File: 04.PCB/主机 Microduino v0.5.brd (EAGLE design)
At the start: 50.8 x 50 mm, 22 parts

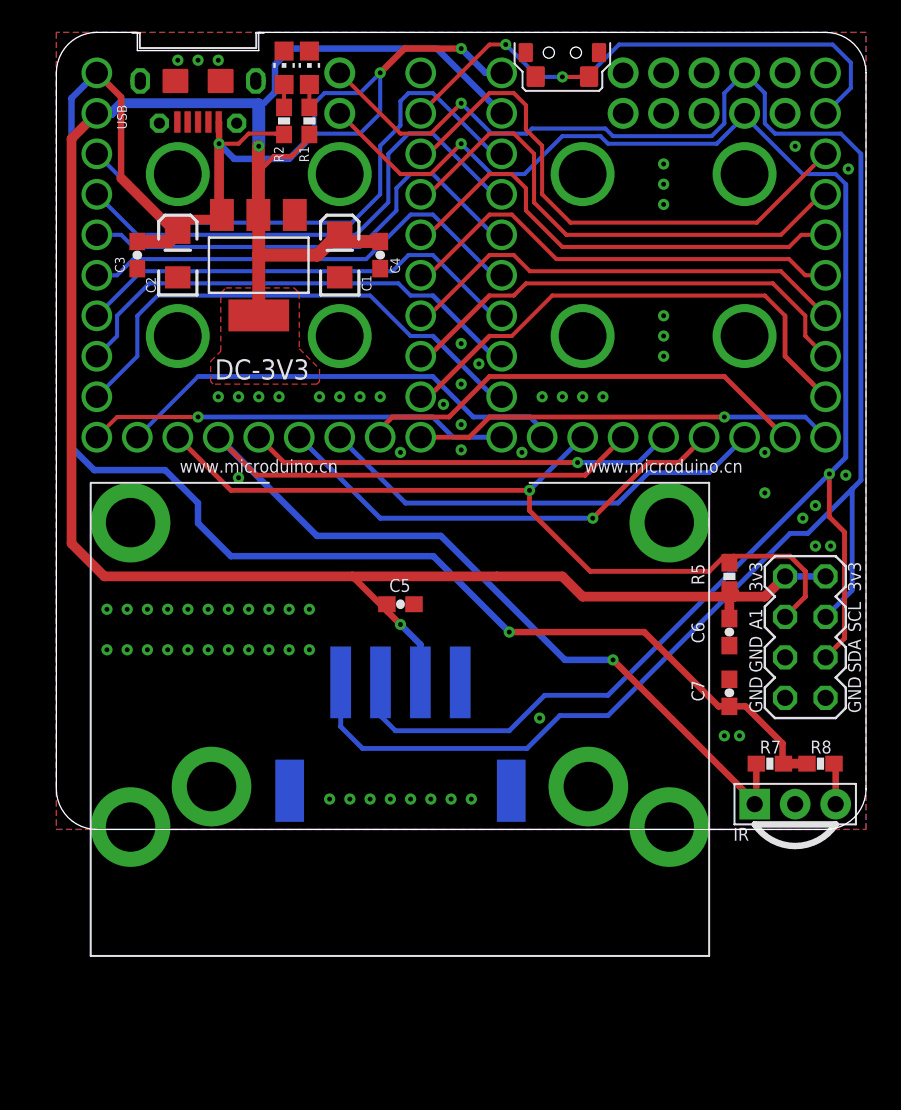
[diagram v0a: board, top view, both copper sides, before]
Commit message: 更新
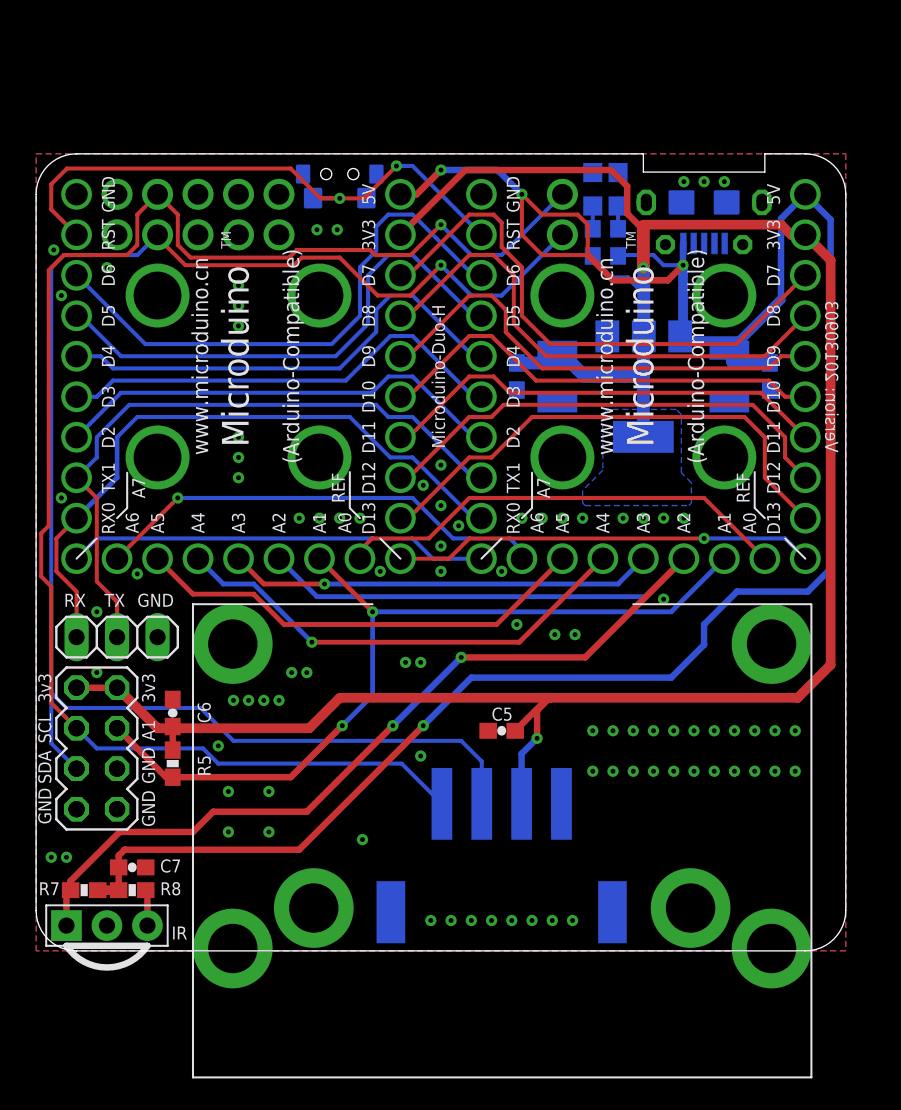
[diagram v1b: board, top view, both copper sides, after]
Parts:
- added JP2: (no value), pinhead:1X03
- added SV1: (no value), pkj:MA04-2
- C1, C2: device microduino:EIA3216 -> microduino:EIA3528
- moved SV2 45.0 mm to (5.71, 15.4), flipped to the bottom
- moved R8 43.9 mm to (7.94, 6.51)
- moved IR 43.8 mm to (6.35, 4.29)
- moved R7 43.7 mm to (4.92, 6.51)
- moved C3 40.4 mm to (47.9, 38.7), flipped to the bottom
- moved C7 39.0 mm to (7.94, 7.94), turned to 0 degrees
- moved R5 36.8 mm to (10.5, 14.4), turned to 90 degrees
- moved C2 35.4 mm to (45.4, 38.7), flipped to the bottom
- moved C6 35.3 mm to (10.5, 17.6), turned to 90 degrees
- moved USB 32.7 mm to (43.8, 49.7), flipped to the bottom
- moved U$2 27.7 mm to (14.6, 50.2), flipped to the bottom
- moved DC-3V3 25.3 mm to (40.0, 38.1), flipped to the bottom
- moved U$1 25.3 mm to (40.0, 50.2), flipped to the bottom
- moved LED2 22.3 mm to (38.4, 50.5), flipped to the bottom
- moved R2 22.3 mm to (38.4, 47.1), flipped to the bottom
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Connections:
- net +3V3: now also SV1.7, SV1.8
- net A1: now also SV1.5
- net D0: now also JP2.1
- net D1: now also JP2.2
- net GND: now also JP2.3, SV1.1, SV1.2, SV1.3
- net SCL: now also SV1.6
- net SDA: now also SV1.4
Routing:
- net SCL: track 114.3 -> 96.3 mm
- net D1: track 29.9 -> 41.0 mm
- net D0: track 32.1 -> 40.7 mm
- net SDA: track 107.1 -> 101.7 mm, vias 4 -> 3
- net A2: track 73.2 -> 77.6 mm, vias 1 -> 2
- net +3V3: track 144.8 -> 146.8 mm
- net +5V: track 139.0 -> 140.1 mm
- net A1: track 53.0 -> 52.8 mm, vias 1 -> 2
- net A6: vias 0 -> 1
- net A7: vias 1 -> 0
- added copper zone on layer 16, net +3V3
- removed copper zone on layer 1, net +3V3
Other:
- outline, holes or cut-outs redrawn
- board text added: "RX"
- board text added: "TX"
- board text added: "Version: 20130903"
- board text removed: "Version: 20130720"
